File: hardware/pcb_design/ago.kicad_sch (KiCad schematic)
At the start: 21 parts

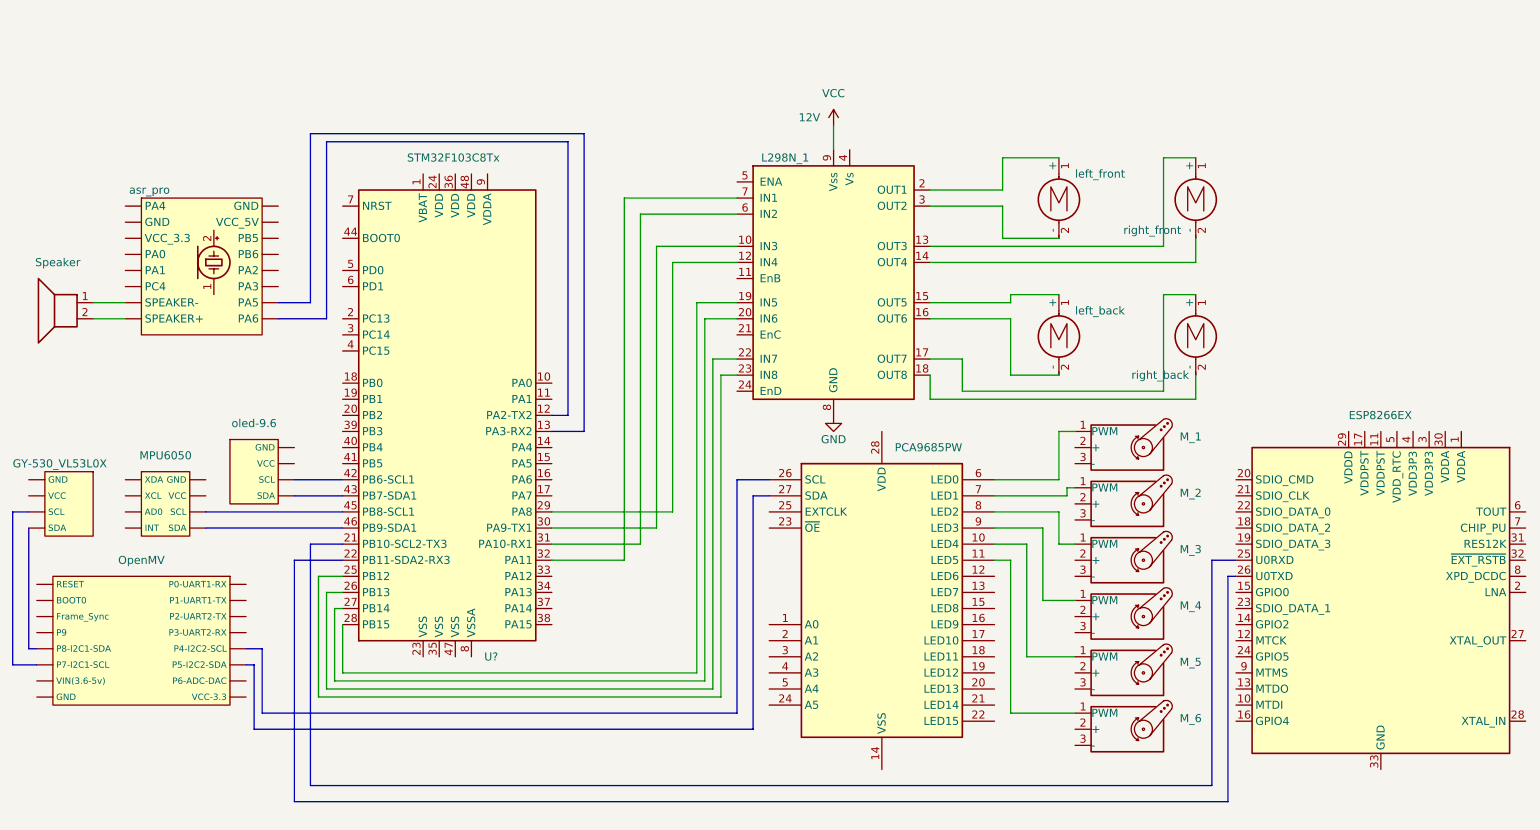
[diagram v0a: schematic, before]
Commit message: refresh hardware design.
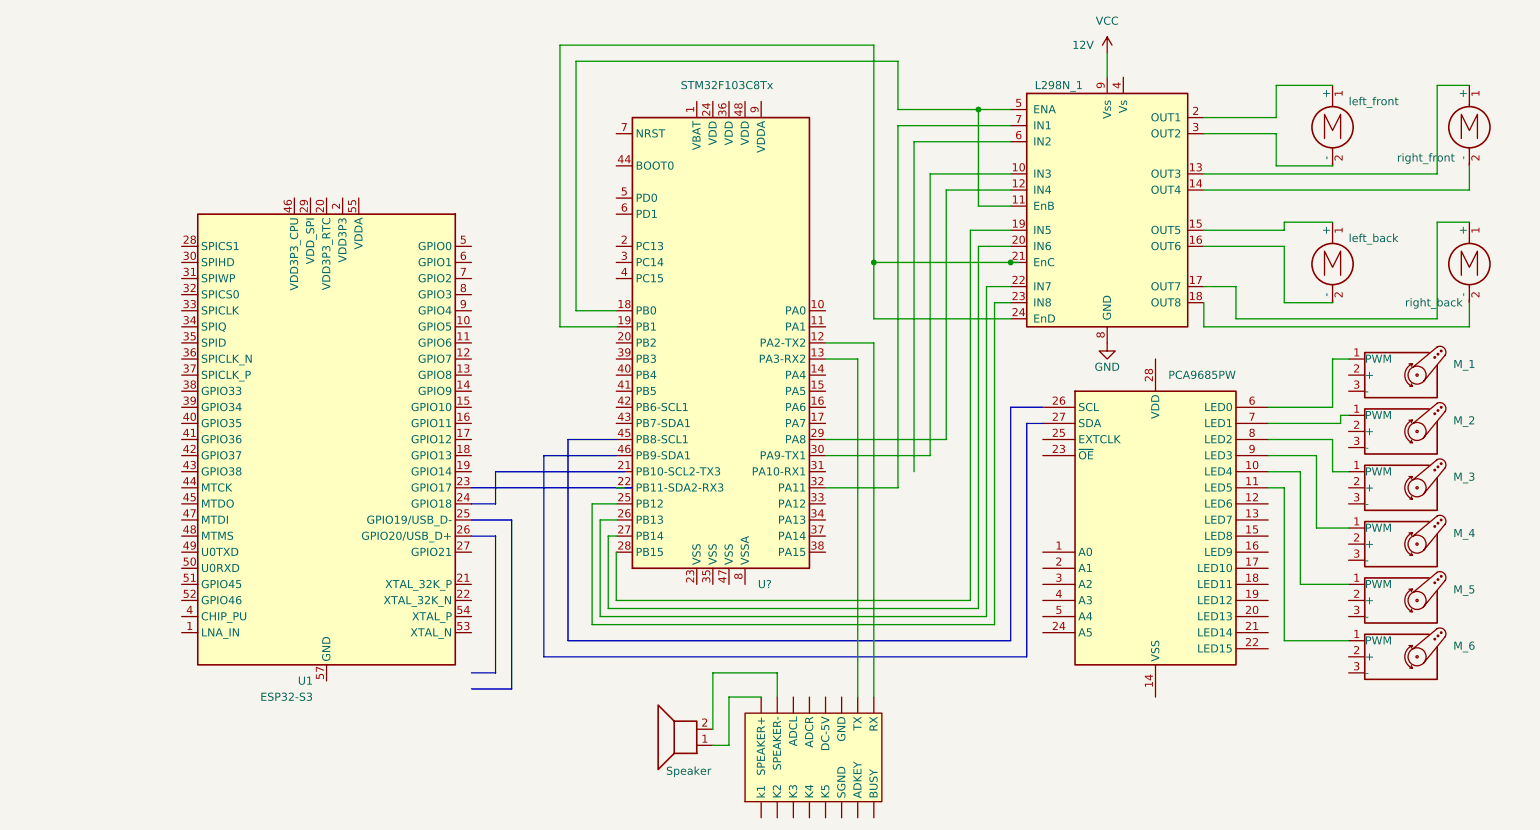
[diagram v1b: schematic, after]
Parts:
- removed MK?: Microphone_Crystal, symbol Device:Microphone_Crystal
- removed U?: OpenMV, symbol Video:OpenMV
- removed U?: ESP8266EX, Package_DFN_QFN:QFN-32-1EP_5x5mm_P0.5mm_EP3.45x3.45mm, symbol MCU_Espressif:ESP8266EX
- removed U?: oled-9.6, symbol Display_Graphic:oled-9.6
- removed U?: MPU6050, symbol Display_Graphic:MPU6050
- removed U?: asr_pro, symbol Device:asr_pro
- removed U?: GY-530_VL53L0X, symbol Video:GY-530_VL53L0X
- added U1: ESP32-S3, Package_DFN_QFN:QFN-56-1EP_7x7mm_P0.4mm_EP4x4mm, symbol MCU_Espressif:ESP32-S3
- added U2: (no value), symbol New_Library:JQ6500
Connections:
- net at LS?.1: now also U2. (RX)
- net at LS?.2: now also U2. (RX)
- net at U?.11 (EnB): now also U?.18 (PB0), U?.5 (ENA)
- net at U?.21 (EnC): now also U?.19 (PB1), U?.24 (EnD)
- net at U?.6 (IN2): no longer U?.31 (PA10-RX1)
- net at U?.12 (PA2-TX2): now also U2. (RX)
- net at U?.13 (PA3-RX2): now also U2. (RX)
- new net: U1.2 (VDD3P3), U1.3 (VDD3P3)
- new net: U1.55 (VDDA), U1.56 (VDDA)
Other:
- moved on the sheet: M_1, M_2, M_3, M_4, M_5, M_6, U?, left_back, left_front, right_back, right_front
